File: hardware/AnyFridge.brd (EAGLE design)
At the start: 160 x 100 mm, 7 parts, among them U1 TSSP77038TT

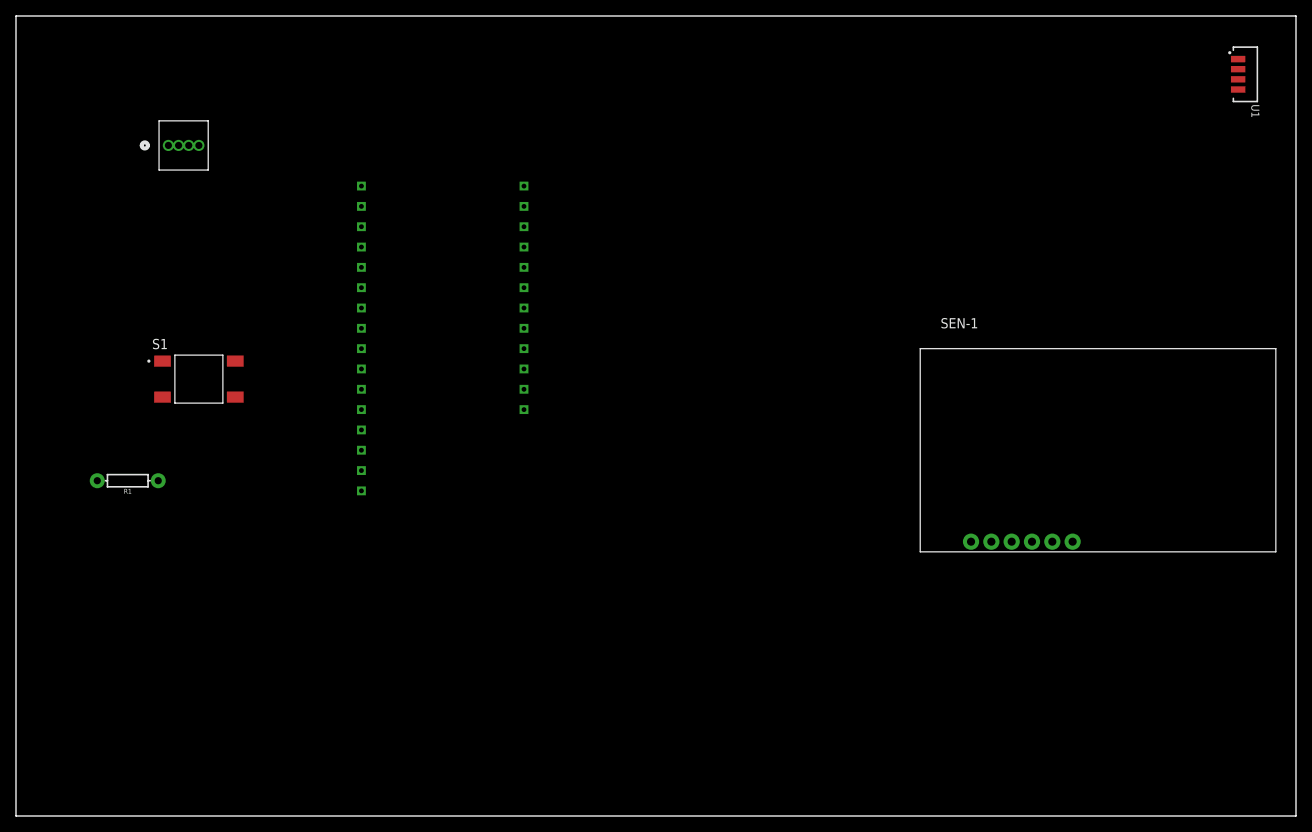
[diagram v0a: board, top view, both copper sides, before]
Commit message: updated board
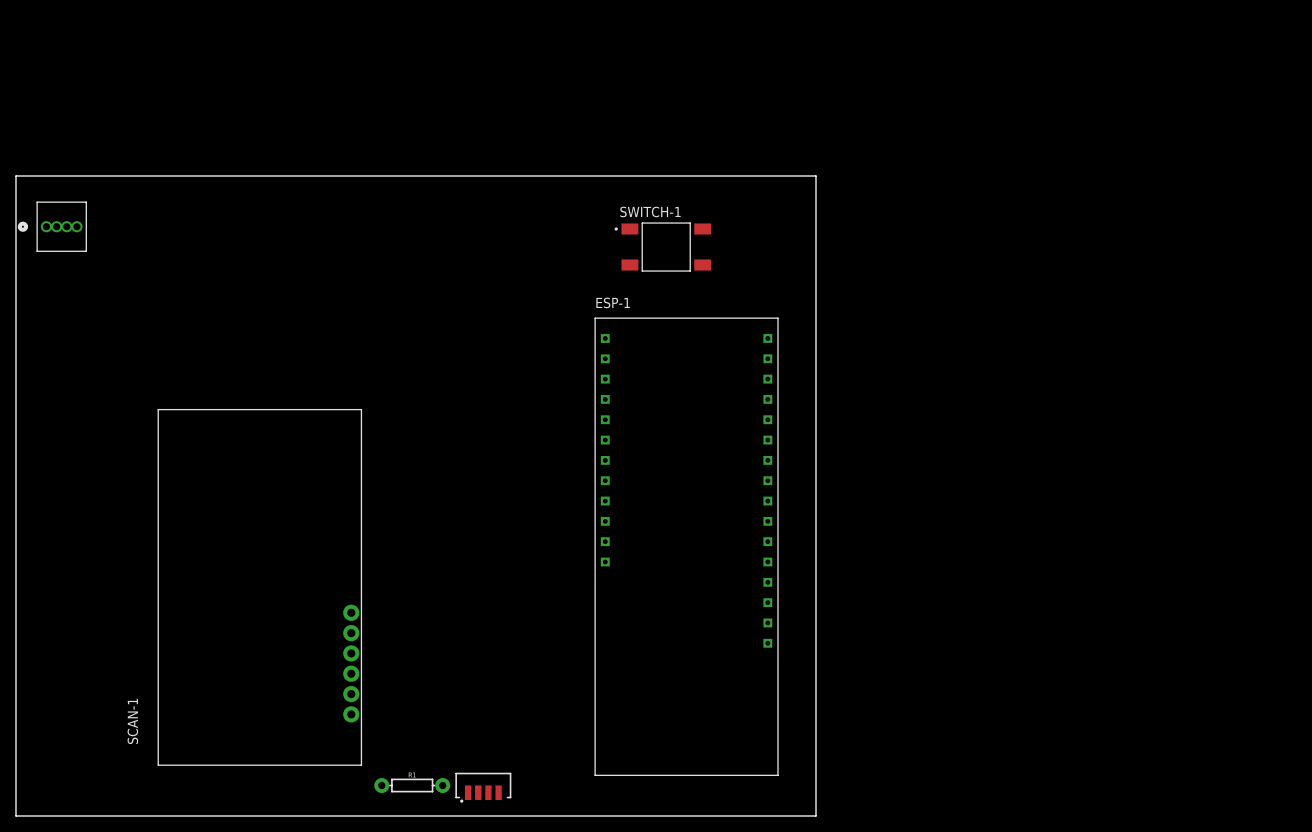
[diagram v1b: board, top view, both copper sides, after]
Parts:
- removed ESP1: ESP32, ESP32:ESP32
- removed LED1: WP154A4SUREQBFZGC, MISC-PARTS:LED4_WP154A4SUREQBFZGC_KNB
- removed S1: TS04-66-73-BK-100-SMT, MISC-PARTS:SW_TS04-66-73-BK-100-SMT
- removed SEN-1: SEN-18088, SEN-18088:SEN-18088
- removed U1: TSSP77038TT, MISC-PARTS:TSSP77038TT
- added ESP-1: ESP32, ESP32:ESP32
- added LED-1: WP154A4SUREQBFZGC, MISC-PARTS:LED4_WP154A4SUREQBFZGC_KNB
- added SCAN-1: SEN-18088, SEN-18088:SEN-18088
- added SENS-1: TSSP77038TT, MISC-PARTS:TSSP77038TT
- added SWITCH-1: TS04-66-73-BK-100-SMT, MISC-PARTS:SW_TS04-66-73-BK-100-SMT
- moved FRAME1 135.5 mm to (43.2, 2.54)
- moved R1 52.1 mm to (49.5, 3.81), turned to 0 degrees
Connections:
- removed net BUTTON: ESP1.15, S1.3
- removed net OUT: ESP1.13, U1.3
- removed net RX0: ESP1.19, SEN-1.RX
- removed net TX0: ESP1.22, SEN-1.TX
- new net RX1: ESP-1.16, SCAN-1.TX
- new net SENS-OUT: ESP-1.13, SENS-1.3
- new net SWI-OUT: ESP-1.15, SWITCH-1.3
- new net TX1: ESP-1.17, SCAN-1.RX
- net 3.3V: now also ESP-1.3V3, SCAN-1.3.3V, SENS-1.2, SWITCH-1.2; no longer ESP1.3V3, S1.2, SEN-1.3.3V, U1.2
- net BLUE: now also ESP-1.12, LED-1.3; no longer ESP1.12, LED1.3
- net GND: now also ESP-1.GND, LED-1.2, SCAN-1.GND, SENS-1.1, SENS-1.4; no longer ESP1.GND, LED1.2, SEN-1.GND, U1.1, U1.4
- net GREEN: now also ESP-1.27, LED-1.4; no longer ESP1.27, LED1.4
- net N$1: now also SWITCH-1.1; no longer S1.1
- net RED: now also ESP-1.33, LED-1.1; no longer ESP1.33, LED1.1
- net STAT: now also ESP-1.23, SCAN-1.STAT; no longer ESP1.23, SEN-1.STAT
- net TRIG: now also ESP-1.21, SCAN-1.TRIG; no longer ESP1.21, SEN-1.TRIG
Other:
- board size 160 x 100 mm -> 100 x 80 mm
